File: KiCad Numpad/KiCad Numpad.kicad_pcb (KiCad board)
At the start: 2 copper layers, 84.9 x 101.6 mm, 36 parts, among them U1 ProMicro

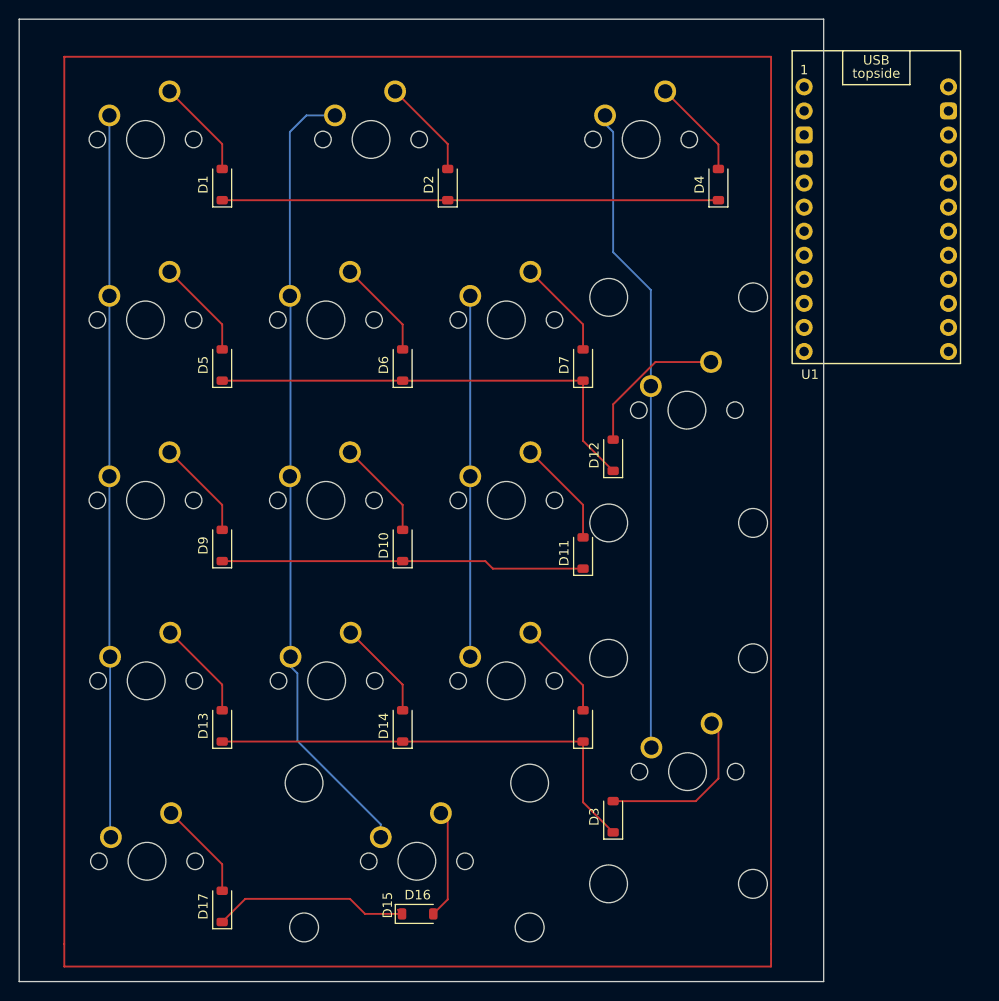
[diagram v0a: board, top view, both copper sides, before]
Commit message: push2
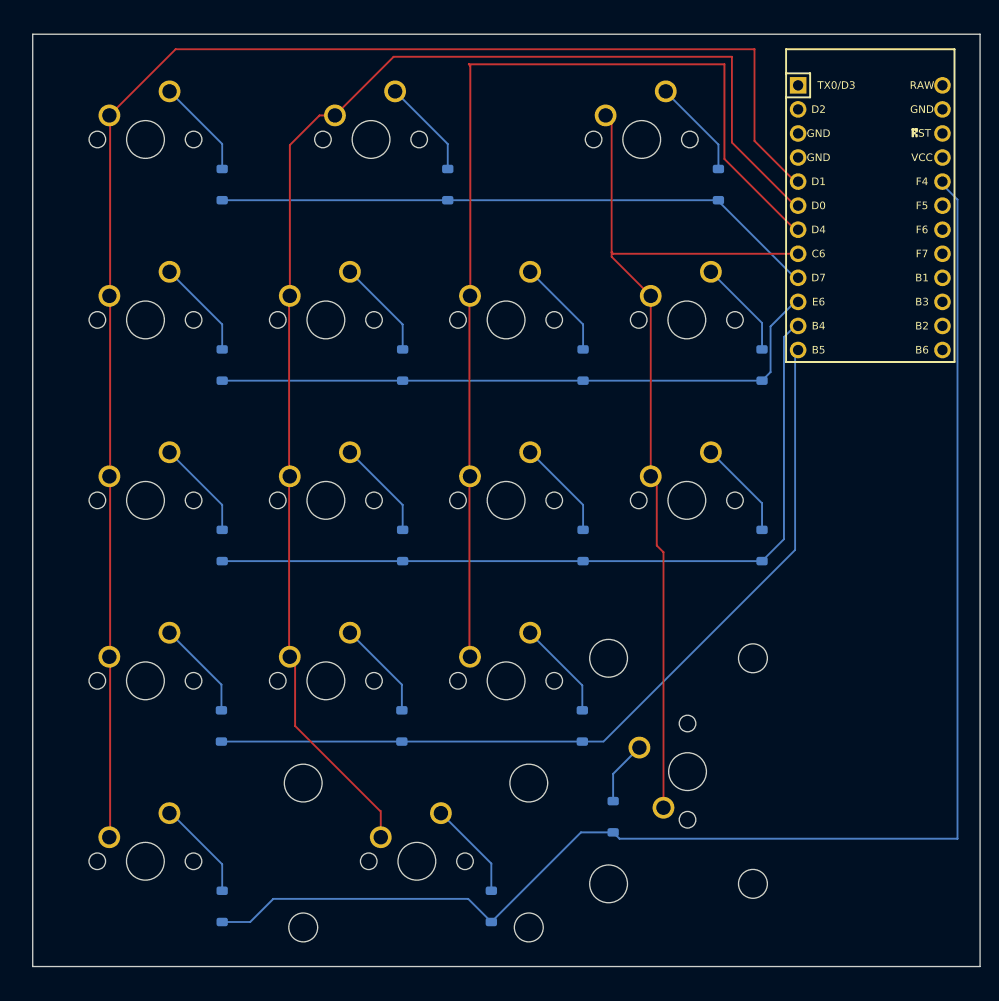
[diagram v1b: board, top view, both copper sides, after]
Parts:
- removed S1: MX_stab, PCM_marbastlib-mx:STAB_MX_2u
- added D8: D_Small, Diode_SMD:D_SOD-123, B.Cu at (169.7, 122.2)
- added MX8: MX_SW_solder, PCM_marbastlib-mx:SW_MX_1u, F.Cu at (161.8, 117.5)
- D1, D10, D11, D12, D13, D14, D15, D16, D17, D2, D3, D4, D5, D6, D7, D9: moved to B.Cu
- S2, S3: moved to F.Cu
- U1: value ProMicro -> Arduino_Pro_Micro; footprint PCM_marbastlib-xp-promicroish:ProMicro_USBup -> ScottoKeebs_MCU:Arduino_Pro_Micro
- moved D12 18.4 mm to (169.7, 103.2)
- moved MX12 9.53 mm to (161.8, 98.4)
- moved D16 7.82 mm to (141.1, 160.3), turned to 90 degrees
- moved D11 0.79 mm to (150.8, 122.2)
- moved U1 0.65 mm to (181.1, 87.6)
- moved MX17 0.17 mm to (104.6, 155.6)
- moved S3 0.09 mm to (133.2, 155.6), turned to 180 degrees
- moved D13 0.08 mm to (112.6, 141.3)
- moved D15 0.08 mm to (150.7, 141.3)
- moved MX13 0.08 mm to (104.6, 136.5)
- moved MX14 0.08 mm to (123.7, 136.5)
- moved D14 0.08 mm to (131.7, 141.3)
- moved MX4 0.06 mm to (157.0, 79.4)
- turned MX3 to 90 degrees
- turned S2 to -90 degrees
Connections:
- D3 pad 1: ROW4 -> ROW5
- U1 pad 10: unconnected-(U1-E6-Pad10) -> ROW2
- U1 pad 11: unconnected-(U1-B4-Pad11) -> ROW3
- U1 pad 12: unconnected-(U1-B5-Pad12) -> ROW4
- U1 pad 20: unconnected-(U1-F7-Pad20) -> ROW5
- U1 pad 23: unconnected-(U1-B2-Pad23) -> GND
- U1 pad 3: unconnected-(U1-GND-Pad3) -> GND
- U1 pad 4: unconnected-(U1-GND-Pad4) -> GND
- U1 pad 5: unconnected-(U1-D1-Pad5) -> COL1
- U1 pad 6: unconnected-(U1-D0-Pad6) -> COL2
- U1 pad 7: unconnected-(U1-D4-Pad7) -> COL3
- U1 pad 8: unconnected-(U1-C6-Pad8) -> COL4
- U1 pad 9: unconnected-(U1-D7-Pad9) -> ROW1
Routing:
- net ROW5: track 21.3 -> 154.0 mm
- net COL1: track 76.7 -> 163.0 mm
- net COL3: track 38.3 -> 110.2 mm
- net COL2: track 85.5 -> 146.1 mm
- net ROW3: track 38.4 -> 83.3 mm
- net ROW4: track 49.0 -> 90.0 mm
- net COL4: track 69.1 -> 95.1 mm
- net ROW2: track 48.9 -> 66.8 mm
- net ROW1: track 52.4 -> 63.9 mm
- net Net-(D3-A): track 18.2 -> 6.80 mm
- net Net-(D8-A): track 0.00 -> 10.4 mm
- net Net-(D12-A): track 15.9 -> 10.4 mm
- net Net-(D16-A): track 11.6 -> 10.4 mm
- net Net-(D11-A): track 11.3 -> 10.5 mm
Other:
- board size 84.9 x 101.6 mm -> 100 x 98.4 mm
